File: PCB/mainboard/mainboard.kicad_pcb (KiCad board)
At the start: 2 copper layers, 22 parts, among them J1 VBuck, J2 Temp, J3 Hall, J4 Display, U1 ATmega8-16A, Y1 16MHz

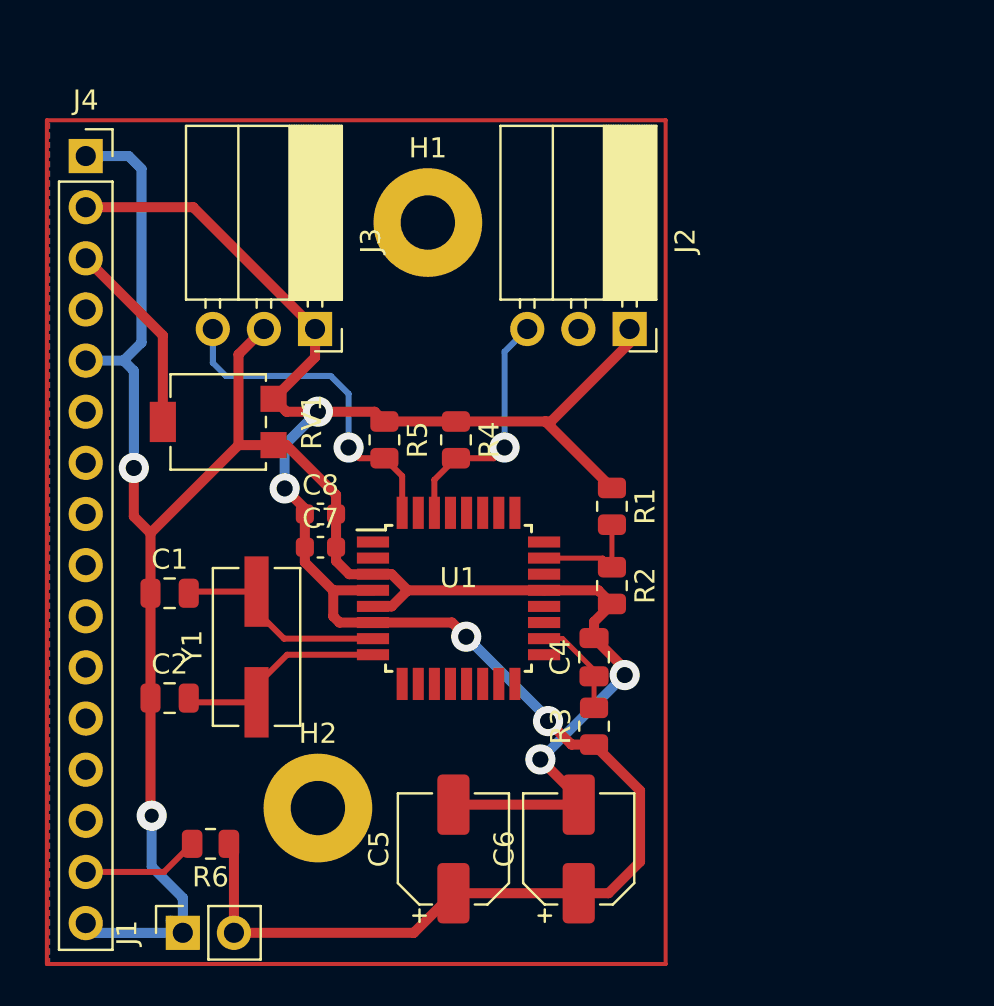
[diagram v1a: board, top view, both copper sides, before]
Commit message: Add files via upload
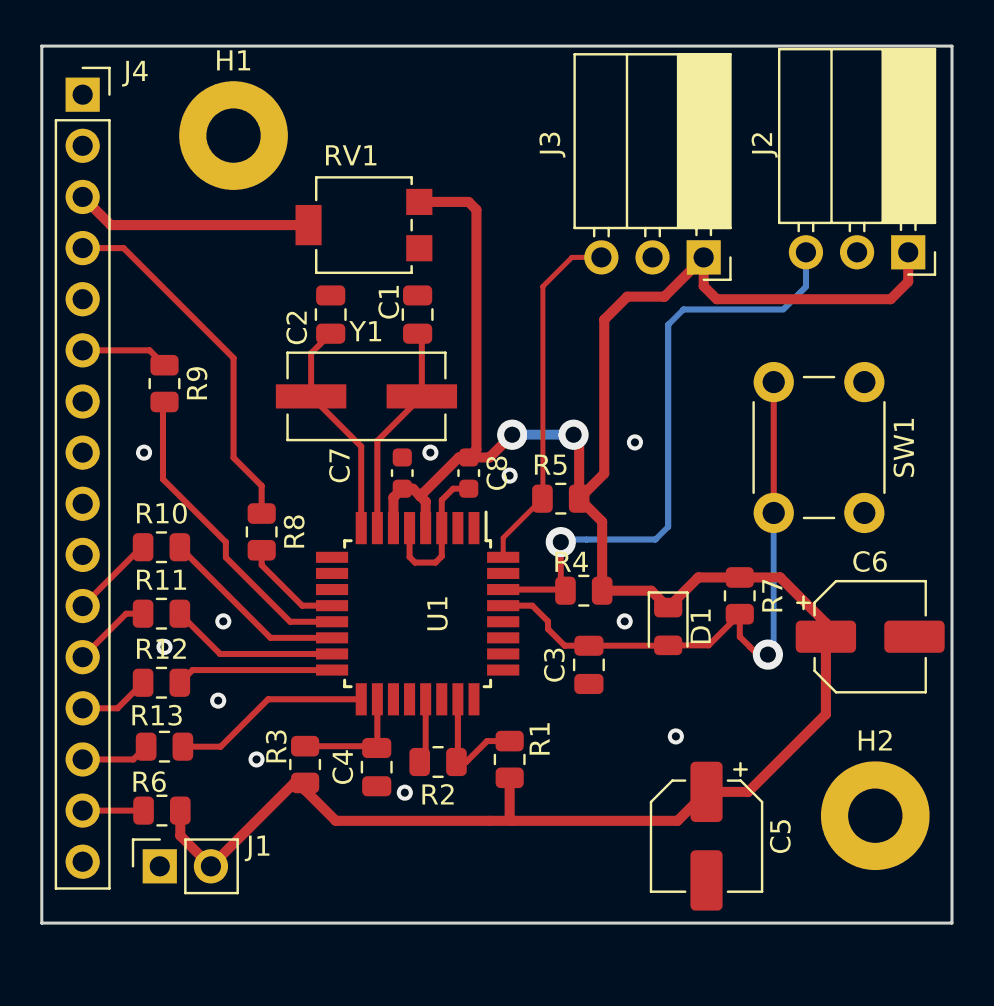
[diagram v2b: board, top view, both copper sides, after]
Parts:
- added C3: 100nF, Capacitor_SMD:C_0805_2012Metric, F.Cu at (135.8, 54.7)
- added D1: D, Diode_SMD:D_0805_2012Metric, F.Cu at (139.7, 52.8)
- added R10: 0, Resistor_SMD:R_0805_2012Metric, F.Cu at (114.5, 48.9)
- added R11: 0, Resistor_SMD:R_0805_2012Metric, F.Cu at (114.5, 52.2)
- added R12: 0, Resistor_SMD:R_0805_2012Metric, F.Cu at (114.5, 55.6)
- added R13: 0, Resistor_SMD:R_0805_2012Metric, F.Cu at (114.7, 58.8)
- added R7: 10k, Resistor_SMD:R_0805_2012Metric, F.Cu at (143.3, 51.3)
- added R8: 0, Resistor_SMD:R_0805_2012Metric, F.Cu at (119.5, 48.1)
- added R9: 0, Resistor_SMD:R_0805_2012Metric, F.Cu at (114.7, 40.8)
- added SW1: SW_Push, Button_Switch_THT:SW_PUSH_6mm, F.Cu at (149.4, 40.7)
- moved H2 27.7 mm to (150.0, 62.2)
- moved C2 20.7 mm to (122.9, 37.3), turned to -90 degrees
- moved J3 19.6 mm to (141.5, 34.5)
- moved C1 18.5 mm to (127.3, 37.3), turned to -90 degrees
- moved C6 17.9 mm to (149.7, 53.3), turned to 0 degrees
- moved R3 14.5 mm to (121.7, 59.7)
- moved J2 14.4 mm to (151.6, 34.2)
- moved Y1 13.6 mm to (124.7, 41.4), turned to 0 degrees
- moved R1 13.6 mm to (131.8, 59.4), turned to 90 degrees
- moved C5 12.6 mm to (141.6, 63.2), turned to -90 degrees
- moved R2 12.3 mm to (128.3, 59.6), turned to 180 degrees
- moved RV1 12.2 mm to (124.6, 32.9)
- moved C4 12.1 mm to (125.2, 59.8), turned to -90 degrees
- moved H1 10.6 mm to (118.1, 28.4)
- moved R4 9.82 mm to (135.5, 51.1), turned to 180 degrees
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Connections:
- C1 pad 1: Vss -> GND
- C2 pad 1: Vss -> GND
- C4 pad 2: Vss -> GND
- C5 pad 2: Vss -> GND
- C6 pad 2: Vss -> GND
- C7 pad 2: Vss -> GND
- C8 pad 2: Vss -> GND
- H1 pad 1: Vss -> GND
- H2 pad 1: Vss -> GND
- J1 pad 1: Vss -> GND
- J2 pad 2: Vss -> GND
- J3 pad 2: Vss -> GND
- J4 pad 11: unconnected-(J4-Pad11) -> Net-(J4-Pad11)
- J4 pad 12: unconnected-(J4-Pad12) -> Net-(J4-Pad12)
- J4 pad 13: unconnected-(J4-Pad13) -> Net-(J4-Pad13)
- J4 pad 14: unconnected-(J4-Pad14) -> Net-(J4-Pad14)
- J4 pad 16: Vss -> GND
- J4 pad 2: VCC -> Vdd
- J4 pad 4: unconnected-(J4-Pad4) -> Net-(J4-Pad4)
- J4 pad 5: Vss -> GND
- J4 pad 6: unconnected-(J4-Pad6) -> Net-(J4-Pad6)
- R2 pad 2: Vss -> GND
- RV1 pad 1: Vss -> GND
- U1 pad 12: unconnected-(U1-Pad12) -> /PB0
- U1 pad 13: unconnected-(U1-Pad13) -> /PB1
- U1 pad 14: unconnected-(U1-Pad14) -> /PB2
- U1 pad 15: unconnected-(U1-Pad15) -> /PB3
- U1 pad 16: unconnected-(U1-Pad16) -> /PB4
- U1 pad 17: unconnected-(U1-Pad17) -> /PB5
- U1 pad 21: Vss -> GND
- U1 pad 29: unconnected-(U1-Pad29) -> RESET
- U1 pad 3: Vss -> GND
- U1 pad 5: Vss -> GND
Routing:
- net Vss: track 108.3 -> 0.00 mm, vias 4 -> 0
- net RESET: track 0.00 -> 30.0 mm, vias 0 -> 1
- net VCC: track 105.8 -> 125.4 mm, vias 4 -> 2
- net Temp: track 12.1 -> 30.6 mm
- net Net-(J4-Pad4): track 0.00 -> 18.1 mm
- net /PB1: track 0.00 -> 15.6 mm
- net GND: track 0.00 -> 10.9 mm, vias 0 -> 11
- net /PB5: track 0.00 -> 9.84 mm
- net /PB2: track 0.00 -> 9.43 mm
- net /PB3: track 0.00 -> 8.39 mm
- net /PB4: track 0.00 -> 7.82 mm
- net /PB0: track 0.00 -> 5.07 mm
- net Net-(J4-Pad6): track 0.00 -> 4.37 mm
- net Net-(J4-Pad11): track 0.00 -> 4.21 mm
- net Net-(J4-Pad12): track 0.00 -> 3.90 mm
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- added copper zone on B.Cu, net GND
- added copper zone on F.Cu, net GND
- removed copper zone on B.Cu, net (none)
- removed copper zone on F.Cu, net (none)
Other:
- board outline added: 45.2 x 43.6 mm
